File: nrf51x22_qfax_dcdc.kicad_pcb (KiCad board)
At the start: 2 copper layers, 14.8 x 16.4 mm, 46 parts, among them U1 nrf51822-qfax, X1 Crystal, X2 XTAL SMD 3.2 x 1.5 mm

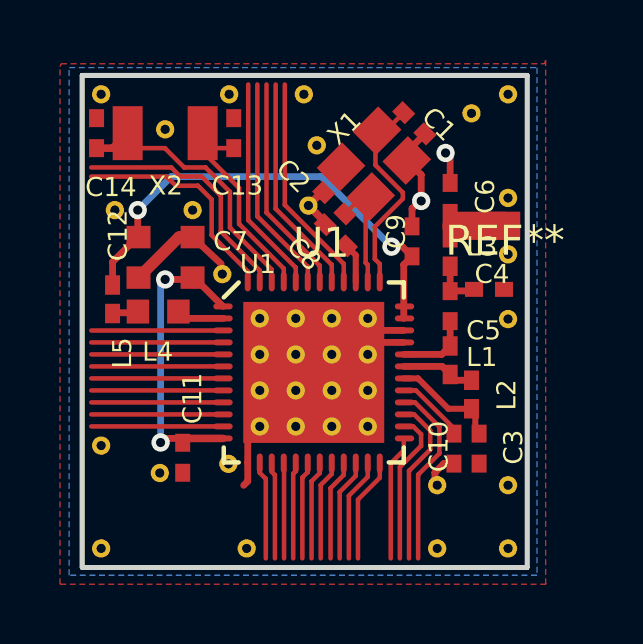
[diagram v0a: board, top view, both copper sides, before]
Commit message: merge library update
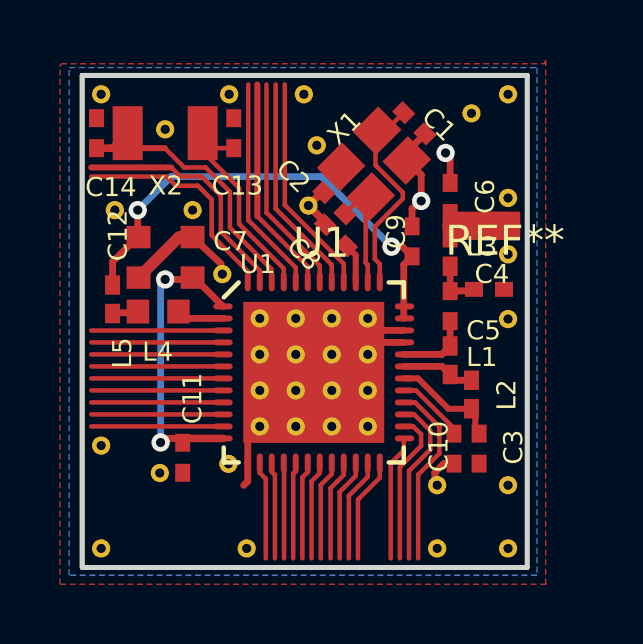
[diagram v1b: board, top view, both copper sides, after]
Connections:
- U1 pad 10: Net-(U1-Pad10) -> (no net)
- U1 pad 11: Net-(U1-Pad11) -> (no net)
- U1 pad 14: Net-(U1-Pad14) -> (no net)
- U1 pad 15: Net-(U1-Pad15) -> (no net)
- U1 pad 16: Net-(U1-Pad16) -> (no net)
- U1 pad 17: Net-(U1-Pad17) -> (no net)
- U1 pad 18: Net-(U1-Pad18) -> (no net)
- U1 pad 19: Net-(U1-Pad19) -> (no net)
- U1 pad 20: Net-(U1-Pad20) -> (no net)
- U1 pad 21: Net-(U1-Pad21) -> (no net)
- U1 pad 22: Net-(U1-Pad22) -> (no net)
- U1 pad 23: Net-(U1-Pad23) -> (no net)
- U1 pad 24: Net-(U1-Pad24) -> (no net)
- U1 pad 25: Net-(U1-Pad25) -> (no net)
- U1 pad 26: Net-(U1-Pad26) -> (no net)
- U1 pad 27: Net-(U1-Pad27) -> (no net)
- U1 pad 28: Net-(U1-Pad28) -> (no net)
- U1 pad 3: Net-(U1-Pad3) -> (no net)
- U1 pad 4: Net-(U1-Pad4) -> (no net)
- U1 pad 40: Net-(U1-Pad40) -> (no net)
- U1 pad 41: Net-(U1-Pad41) -> (no net)
- U1 pad 42: Net-(U1-Pad42) -> (no net)
- U1 pad 43: Net-(U1-Pad43) -> (no net)
- U1 pad 44: Net-(U1-Pad44) -> (no net)
- U1 pad 45: Net-(U1-Pad45) -> (no net)
- U1 pad 46: Net-(U1-Pad46) -> (no net)
- U1 pad 47: Net-(U1-Pad47) -> (no net)
- U1 pad 48: Net-(U1-Pad48) -> (no net)
- U1 pad 5: Net-(U1-Pad5) -> (no net)
- U1 pad 6: Net-(U1-Pad6) -> (no net)
- U1 pad 7: Net-(U1-Pad7) -> (no net)
- U1 pad 8: Net-(U1-Pad8) -> (no net)
- U1 pad 9: Net-(U1-Pad9) -> (no net)
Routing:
- net (no net): track 0.00 -> 149.8 mm
- net Net-(U1-Pad47): track 8.14 -> 0.00 mm
- net Net-(U1-Pad48): track 7.59 -> 0.00 mm
- net Net-(U1-Pad40): track 7.41 -> 0.00 mm
- net Net-(U1-Pad41): track 7.37 -> 0.00 mm
- net Net-(U1-Pad42): track 7.33 -> 0.00 mm
- net Net-(U1-Pad43): track 7.29 -> 0.00 mm
- net Net-(U1-Pad44): track 7.26 -> 0.00 mm
- net Net-(U1-Pad28): track 6.20 -> 0.00 mm
- net Net-(U1-Pad27): track 5.66 -> 0.00 mm
- net Net-(U1-Pad26): track 5.12 -> 0.00 mm
- net Net-(U1-Pad9): track 4.42 -> 0.00 mm
- net Net-(U1-Pad8): track 4.42 -> 0.00 mm
- net Net-(U1-Pad7): track 4.42 -> 0.00 mm
- net Net-(U1-Pad6): track 4.42 -> 0.00 mm
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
